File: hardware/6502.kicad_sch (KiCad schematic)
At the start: 82 parts, among them J1 5V, J10 JMP, J12 Control_bus, J14 Power, J15 Data_bus, J16 Address bus, J17 USB_A, J2 PORTAB, J20 Interface, J3 CA, J4 CB, J5 W27c512?, J8 5V, J9 USB_B_Micro, SW1 SW_Push, U1 74HC14, U13 74HC74, U14 74HC04, U15 MIC5504-3.3YM5, U17 74HC00, U2 R6502, U21 74HC00, U3 R6522, U4 74HC273, U5 SST39SF010, U8 74HC32, U9 NRF24L01_Breakout

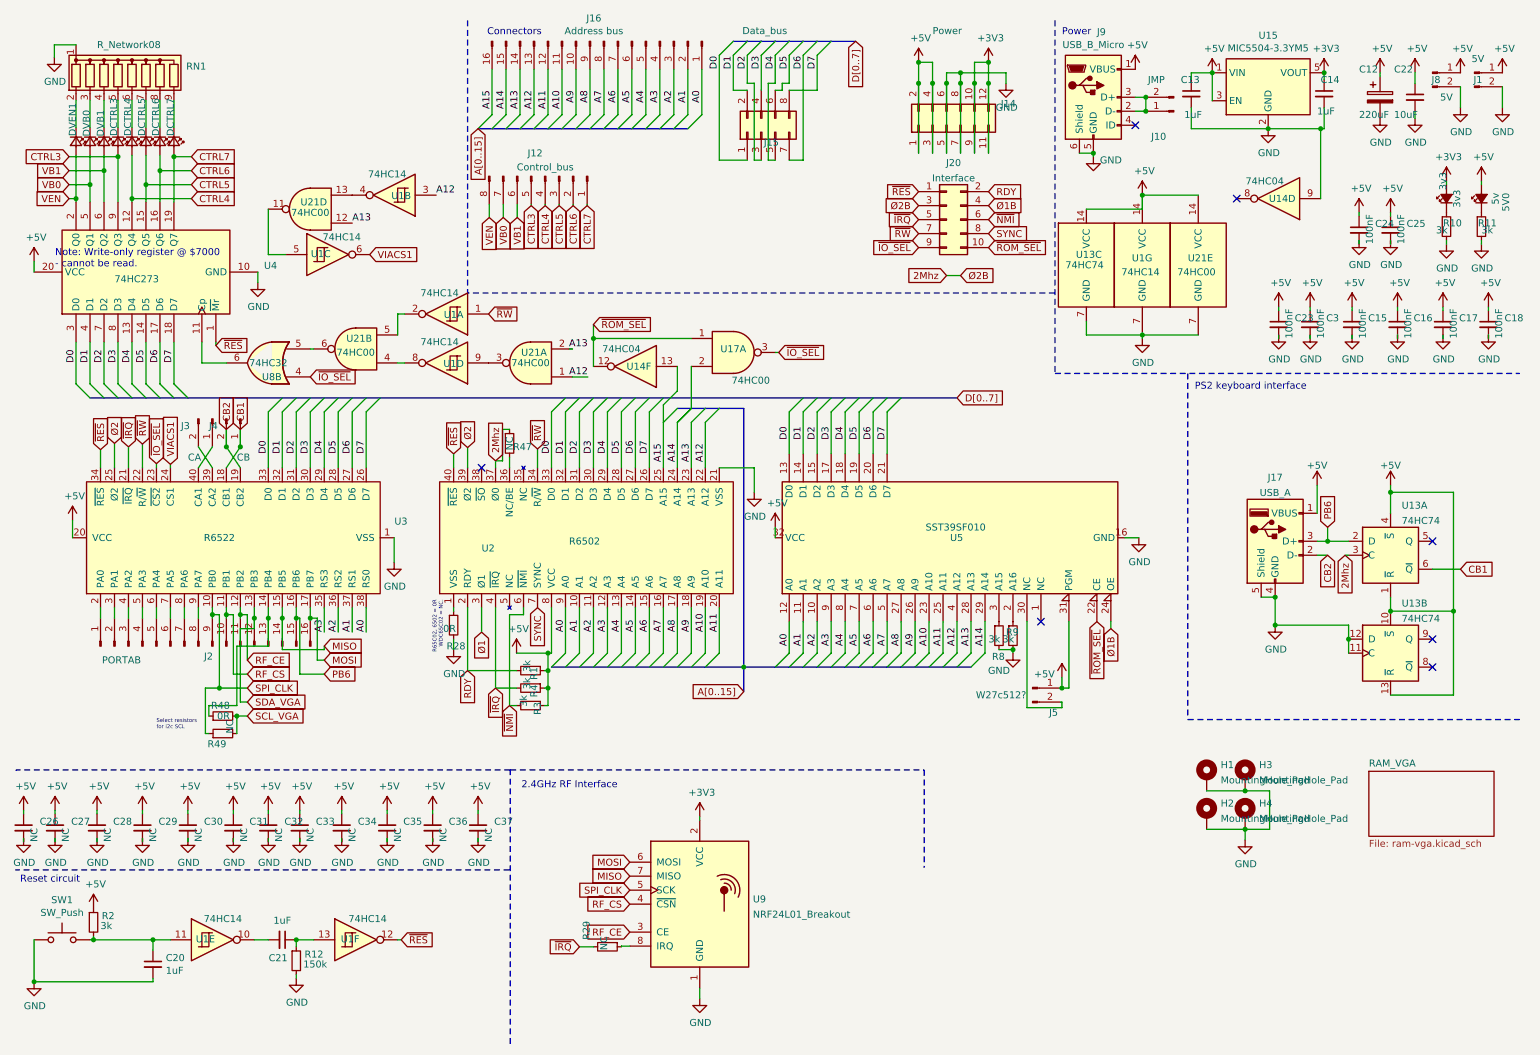
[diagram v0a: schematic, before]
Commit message: Revision 2 published
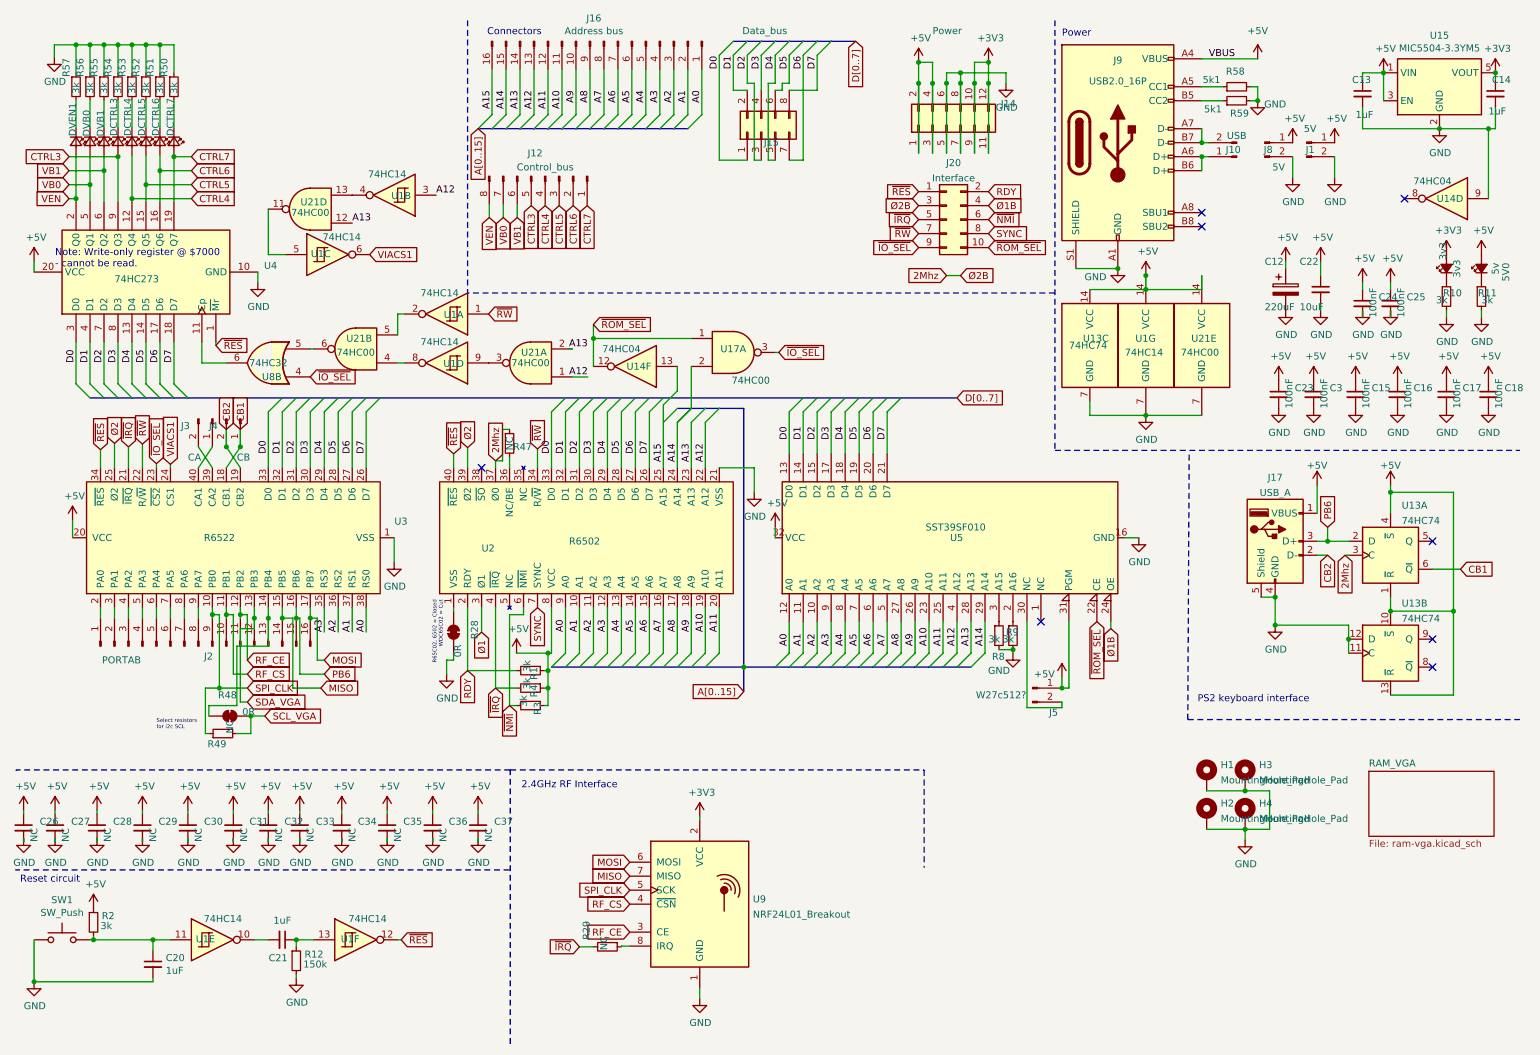
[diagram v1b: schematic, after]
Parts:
- removed J9: USB_B_Micro, Connector_USB:USB_Micro-B_Amphenol_10118194_Horizontal, symbol 6502-rescue:USB_B_Micro-Connector
- removed R48: 0R, Resistor_SMD:R_0805_2012Metric, symbol Device:R_Small
- removed RN1: R_Network08, Resistor_THT:R_Array_SIP9, symbol Device:R_Network08
- added J9: USB2.0_16P, Connector_USB:USB_C_Receptacle_HCTL_HC-TYPE-C-16P-01A, symbol Connector:USB_C_Receptacle_USB2.0_16P
- added R48: 0R, Jumper:SolderJumper-2_P1.3mm_Bridged_RoundedPad1.0x1.5mm, symbol Jumper:SolderJumper_2_Bridged
- added R50, R51, R52, R53, R54, R55, R56, R57: 3k, Resistor_SMD:R_0805_2012Metric, symbol Device:R_Small
- added R58, R59: 5k1, Resistor_SMD:R_0805_2012Metric, symbol Device:R_Small
- C13, C14, C20, C21: LCSC (none) -> C28323
- C15, C16, C17, C18, C23, C24, C25, C3: LCSC (none) -> C14663
- J10: value JMP -> USB
- J14: LCSC (none) -> C92269
- J15: LCSC (none) -> C92271
- J16: LCSC (none) -> C30734
- J17: LCSC (none) -> C456018
- J2: LCSC (none) -> C7500783
- J20: LCSC (none) -> C2685204
- J3, J4: LCSC (none) -> C7499322
- R1, R10, R11, R2, R3, R4, R8, R9: LCSC (none) -> C17661
- R12: LCSC (none) -> C17470
- R28: footprint Jumper:SolderJumper-2_P1.3mm_Open_RoundedPad1.0x1.5mm -> Jumper:SolderJumper-2_P1.3mm_Bridged_RoundedPad1.0x1.5mm; symbol Device:R_Small -> Jumper:SolderJumper_2_Bridged; now left out of the parts list
- U1, U13, U14, U17, U21, U8: LCSC (none) -> C2325
- U2, U3: LCSC (none) -> C72123
- U4: LCSC (none) -> C72118
- U5: LCSC (none) -> C146583
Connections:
- net +5V: now also J9.A4 (VBUS), J9.A9 (VBUS), J9.B4 (VBUS), J9.B9 (VBUS)
- net GND: now also R28.1 (A), J9.A1 (GND), J9.A12 (GND), J9.B1 (GND), J9.B12 (GND), J9.S1 (SHIELD), R50.1, R51.1, R52.1, R53.1, R54.1, R55.1, R56.1, R57.1, R58.2, R59.2; no longer R28.2
- net SCL_VGA: now also R48.1 (A)
- net at U2.1 (VSS): now also R28.2 (B); no longer R28.1
- net at DVEN1.1 (K): now also R57.2
- net at DVB0.1 (K): now also R56.2
- net at DVB1.1 (K): now also R55.2
- net at DCTRL3.1 (K): now also R54.2
- net at DCTRL4.1 (K): now also R53.2
- net at DCTRL5.1 (K): now also R52.2
- net at DCTRL6.1 (K): now also R51.2
- net at DCTRL7.1 (K): now also R50.2
- net at J2.13 (Pin_13), U3.14 (PB4): now also R48.2 (B)
- net at J10.1 (Pin_1): now also J9.A6 (D+), J9.B6 (D+); no longer J10.2 (Pin_2)
- new net: J9.B5 (CC2), R59.1
- new net: J9.A5 (CC1), R58.1
- new net: J10.2 (Pin_2), J9.A7 (D-), J9.B7 (D-)
- no-connect marks 7 -> 8
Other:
- note added: "R65C02, 6502 = Closed WDC65C02 = Cut"
- note removed: "R65C02, 6502 = 0R WDC65C02 = NC."
- title: ABNielsen.com 6502 Single Board Computer R1 B4 -> ABNielsen.com 6502 Single Board Computer Rev. 2
- moved on the sheet: 3v3, 5V0, C12, C13, C14, C15, C16, C17, C18, C22, C23, C24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
